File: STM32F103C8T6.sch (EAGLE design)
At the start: 40 parts, among them IC1 MCP170333MB, J1 455-1750-1-ND, J2 455-1750-1-ND, J4 CORTEX_DEBUG_MINIMUM_PTH, U1 STM32F103C8T6, Y2 32.768kHz

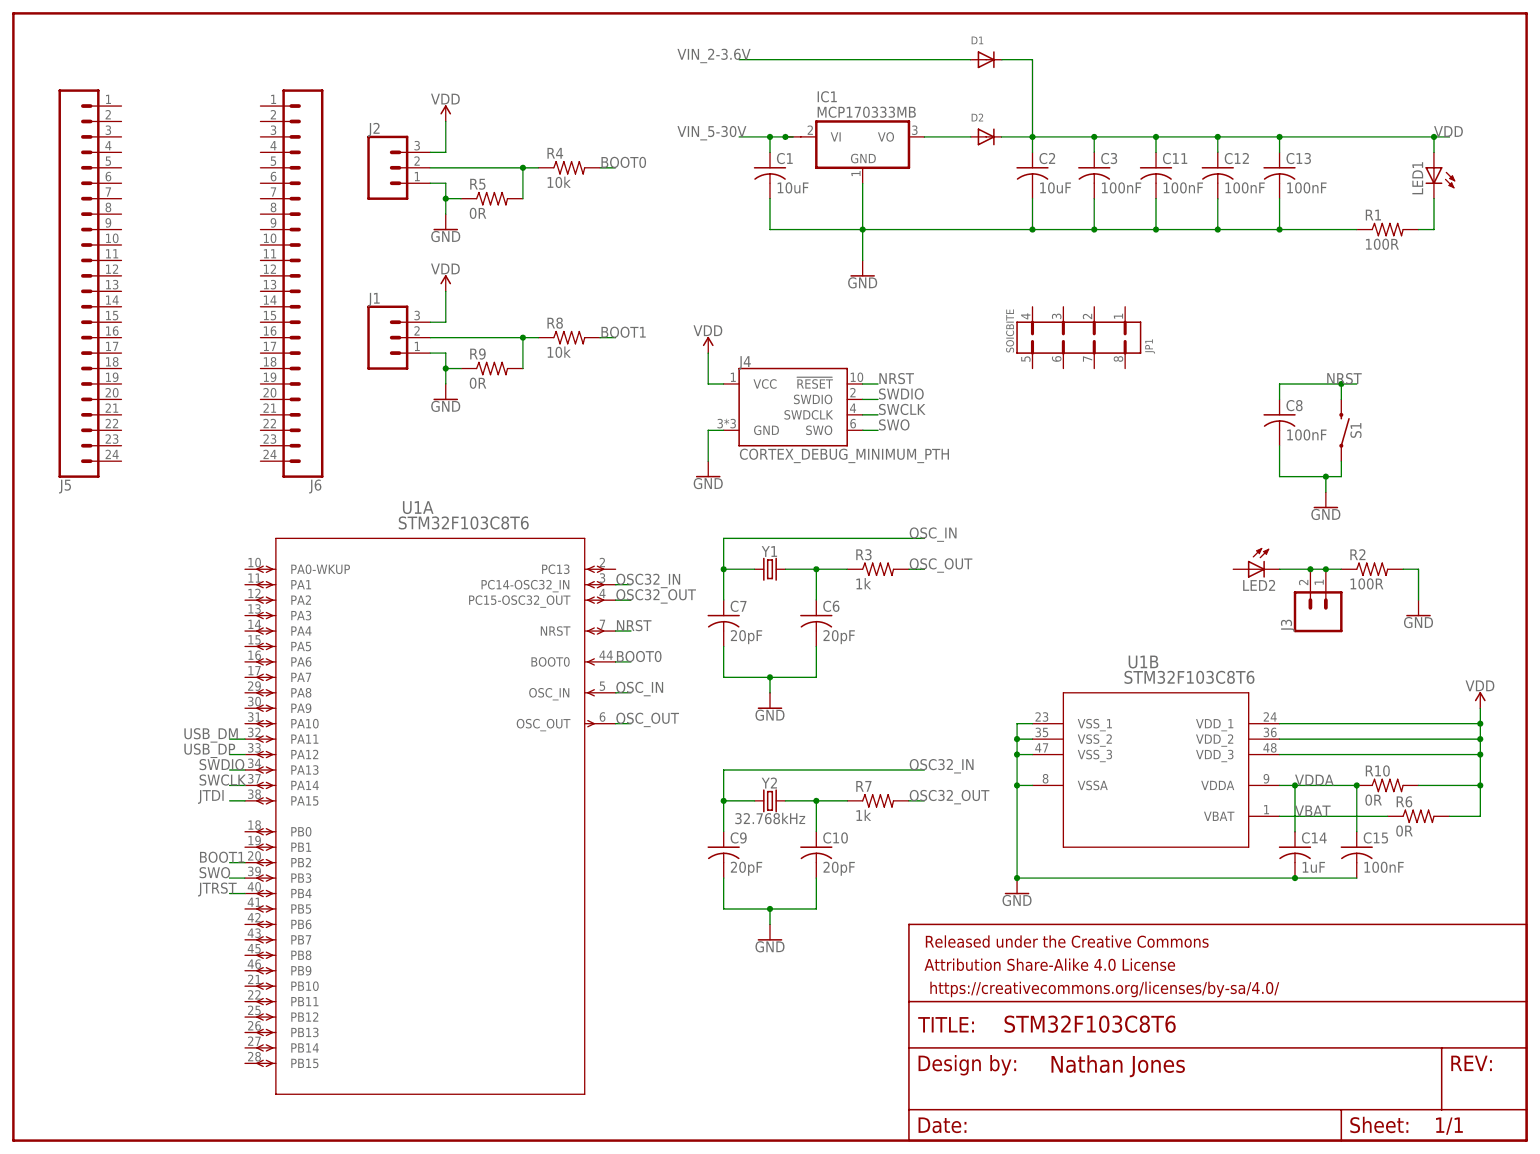
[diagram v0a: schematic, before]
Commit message: Nearly finalized circuit.
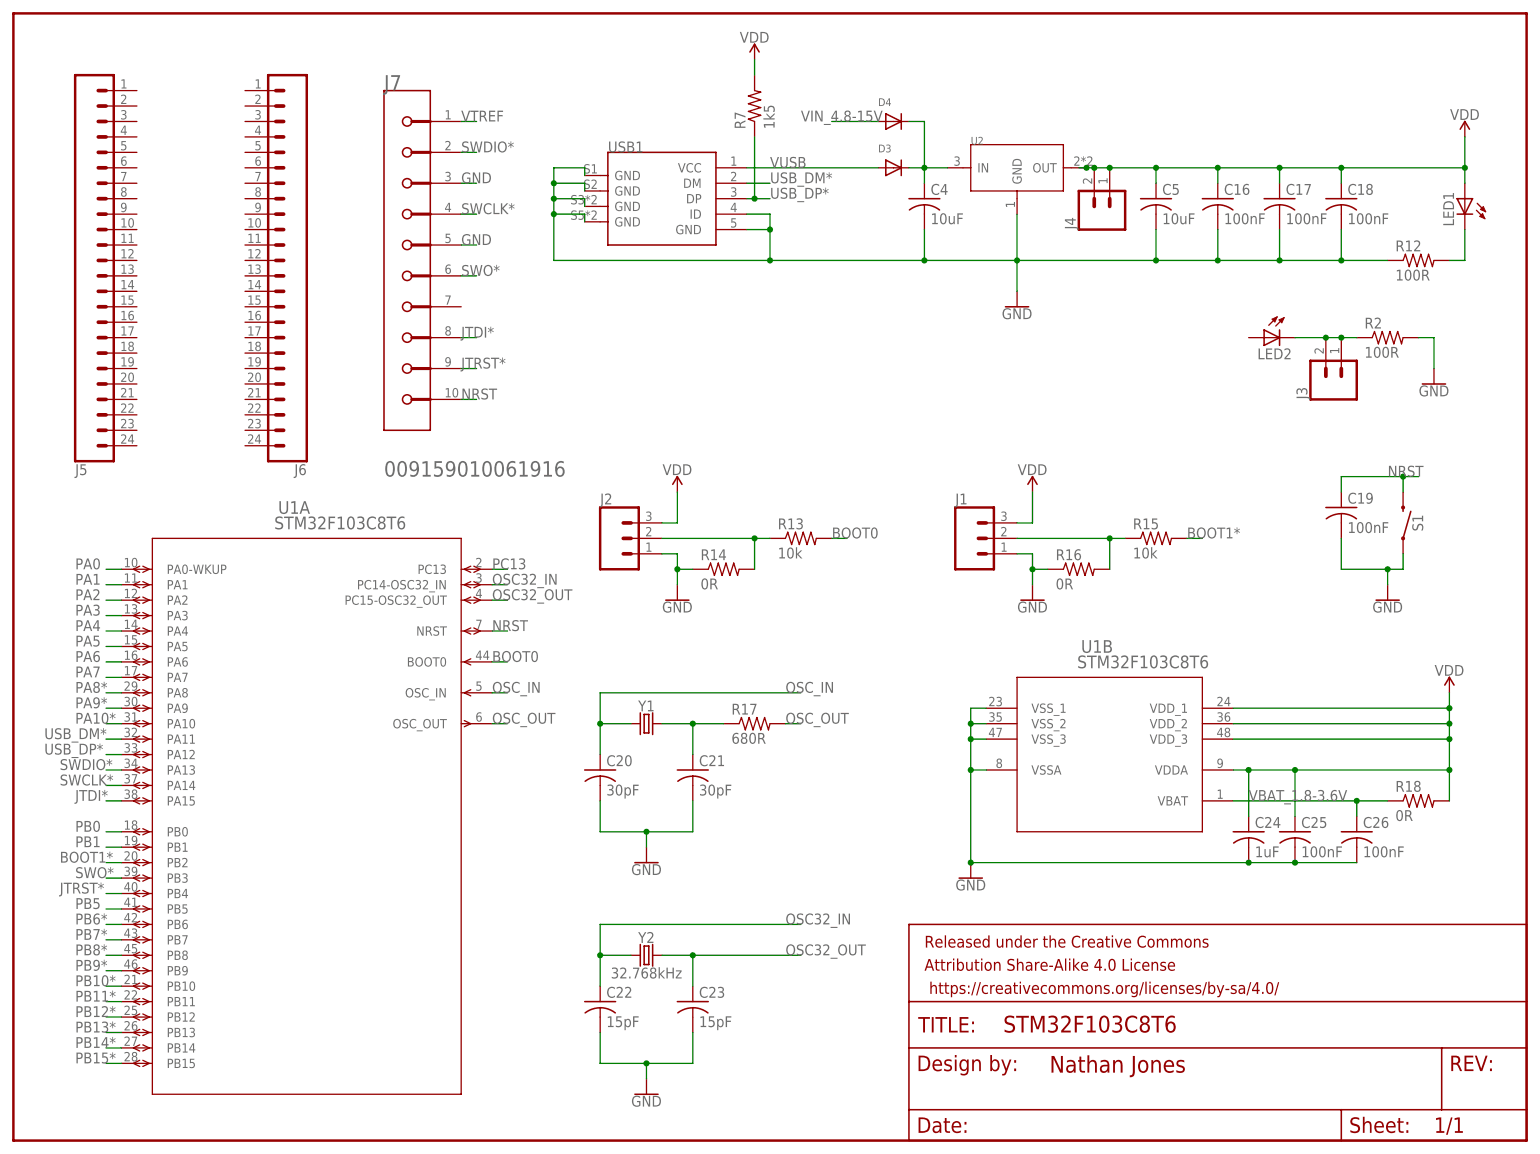
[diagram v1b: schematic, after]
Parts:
- removed C1, C2: 10uF, adafruit:C-USC0603
- removed C10, C6, C7, C9: 20pF, adafruit:C-USC0603
- removed C11, C12, C13, C15, C3, C8: 100nF, adafruit:C-USC0603
- removed C14: 1uF, adafruit:C-USC0603
- removed D1, D2: (no value), adafruit:DIODESOD-123
- removed IC1: MCP170333MB, linear:MCP170333MB
- removed JP1: SOICBITE, SOICbite_Eagle:SOICBITE
- removed R1: 100R, adafruit:R-US_R0603
- removed R10, R5, R6, R9: 0R, adafruit:R-US_R0603
- removed R3: 1k, adafruit:R-US_R0603
- removed R4, R8: 10k, adafruit:R-US_R0603
- added C16, C17, C18, C19, C25, C26: 100nF, adafruit:C-USC0402
- added C20, C21: 30pF, adafruit:C-USC0402
- added C22, C23: 15pF, adafruit:C-USC0402
- added C24: 1uF, adafruit:C-USC0402
- added C4, C5: 10uF, adafruit:C-USC0402
- added D3, D4: (no value), adafruit:DIODESOD-123
- added J7: AVX_009159010061916AVX_009159010061916_0_0, AVX - 009159010061916:AVX_009159010061916AVX_009159010061916_0_0
- added R12: 100R, adafruit:R-US_R0402
- added R13, R15: 10k, adafruit:R-US_R0402
- added R14, R16, R18: 0R, adafruit:R-US_R0402
- added R17: 680R, adafruit:R-US_R0402
- added U2: CJT1117-3.3-SOT223, OPL_IC:PMIC-CJT1117-3.3(SOT223)
- added USB1: 10118193-0001LF, OPL_Connector:MICRO-USB-SMD-B-(10118193-0001LF)
- J4: value CORTEX_DEBUG_MINIMUM_PTH -> (none); device SparkFun-Connectors:CORTEX_DEBUG_MINIMUM_PTH -> SparkFun-Connectors:CONN_02
- R7: value 1k -> 1k5; device adafruit:R-US_R0603 -> adafruit:R-US_R0402
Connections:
- removed net BOOT1: R8.2, U1A.PB2
- removed net JTDI: U1A.PA15
- removed net JTRST: U1A.PB4
- removed net N$4: C10.1, R7.1, Y2.2
- removed net N$5: D2.A, IC1.VO
- removed net SWCLK: J4.SWDCLK, U1A.PA14
- removed net SWDIO: J4.SWDIO, U1A.PA13
- removed net SWO: J4.SWO, U1A.PB3
- removed net USB_DM: U1A.PA11
- removed net USB_DP: U1A.PA12
- removed net VBAT: R6.1, U1B.VBAT
- removed net VDDA: C14.1, C15.1, R10.1, U1B.VDDA
- removed net VIN_2-3.6V: D1.A
- removed net VIN_5-30V: C1.1, IC1.VI1
- new net BOOT1*: R15.2, U1A.PB2
- new net JTDI*: J7.8, U1A.PA15
- new net JTRST*: J7.9, U1A.PB4
- new net PA0: U1A.PA0-WKUP
- new net PA1: U1A.PA1
- new net PA10*: U1A.PA10
- new net PA2: U1A.PA2
- new net PA3: U1A.PA3
- new net PA4: U1A.PA4
- new net PA5: U1A.PA5
- new net PA6: U1A.PA6
- new net PA7: U1A.PA7
- new net PA8*: U1A.PA8
- new net PA9*: U1A.PA9
- new net PB0: U1A.PB0
- new net PB1: U1A.PB1
- new net PB10*: U1A.PB10
- new net PB11*: U1A.PB11
- new net PB12*: U1A.PB12
- new net PB13*: U1A.PB13
- new net PB14*: U1A.PB14
- new net PB15*: U1A.PB15
- new net PB5: U1A.PB5
- new net PB6*: U1A.PB6
- new net PB7*: U1A.PB7
- new net PB8*: U1A.PB8
- new net PB9*: U1A.PB9
- new net PC13: U1A.PC13
- new net SWCLK*: J7.4, U1A.PA14
- new net SWDIO*: J7.2, U1A.PA13
- new net SWO*: J7.6, U1A.PB3
- new net USB_DM*: U1A.PA11, USB1.DM
- new net USB_DP*: R7.1, U1A.PA12, USB1.DP
- new net VBAT_1.8-3.6V: C26.1, R18.1, U1B.VBAT
- new net VIN: C4.1, D3.C, D4.C, U2.IN
- new net VIN_4.8-15V: D4.A
- new net VTREF: J7.1
- new net VUSB: D3.A, USB1.VCC
- net BOOT0: now also R13.2; no longer R4.2
- net GND: now also C16.2, C17.2, C18.2, C19.2, C20.2, C21.2, C22.2, C23.2, C24.2, C25.2, C26.2, C4.2, C5.2, J7.3, J7.5, R12.1, R14.1, R16.1, U2.GND, USB1.GND@1, USB1.GND@2, USB1.GND@3, USB1.GND@4, USB1.GND@5, USB1.ID; no longer C1.2, C10.2, C11.2, C12.2, C13.2, C14.2, C15.2, C2.2, C3.2, C6.2, C7.2, C8.2, C9.2, IC1.GND, J4.GND, R1.1, R5.1, R9.1
- net N$1: now also R13.1, R14.2; no longer R4.1, R5.2
- net N$3: now also C21.1, R17.1; no longer C6.1, R3.1
- net N$6: now also R15.1, R16.2; no longer R8.1, R9.2
- net N$7: now also R12.2; no longer R1.2
- net NRST: now also C19.1, J7.10; no longer C8.1, J4.!RESET
- net OSC32_IN: now also C22.1; no longer C9.1
- net OSC32_OUT: now also C23.1, Y2.2; no longer R7.2
- net OSC_IN: now also C20.1; no longer C7.1
- net OSC_OUT: now also R17.2; no longer R3.2
- net VDD: now also C16.1, C17.1, C18.1, C24.1, C25.1, C5.1, J4.1, J4.2, R18.2, R7.2, U1B.VDDA, U2.OUT; no longer C11.1, C12.1, C13.1, C2.1, C3.1, D1.C, D2.C, J4.VCC, R10.2, R6.2
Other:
- moved on the sheet: J1, J2, J3, J5, J6, LED1, LED2, R2, R7, S1, U1A, U1B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
